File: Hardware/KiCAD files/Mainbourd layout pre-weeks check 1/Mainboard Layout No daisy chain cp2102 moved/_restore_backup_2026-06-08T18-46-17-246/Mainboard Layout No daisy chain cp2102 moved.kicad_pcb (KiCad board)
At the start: 2 copper layers, 207 x 174.8 mm, 107 parts, among them J1 JST_03, J11 Conn_01x04, J12 JST_06, J13 Conn_01x08, J14 Conn_01x08, J17 PINHD_1x8_Male, J18 PINHD_1x8_Male, J19 PINHD_1x8_Male, J2 Screw_Terminal_2_P5.00mm, J20 PINHD_1x8_Male, J22 PINHD_1x8_Male, J23 PINHD_1x8_Male, J24 PINHD_1x8_Male, J25 Conn_01x04, J26 Conn_01x04, J27 Conn_01x04, J28 PINHD_1x8_Male, J3 Screw_Terminal_2_P3.50mm, J30 USB-A1VSB6, J31 JST_03, J32 USB-A1VSB6, J34 JST_03, J35 JST_03, J36 JST_03, J37 JST_03, J38 JST_03, J4 JST_06, J5 Conn_01x04, J6 JST_06, J7 JST_06, J9 Conn_01x10, Q1 BS170, Q2 2DD1664, SW1 210-4MS, SW2 210-4MS, SW3 210-4MS, SW4 210-4MS, SW8 Push_Button, SW9 Push_Button, U1 CP2102-GM, U12 ESP32-S3-WROOM-1, U2 PCA9534PW_118, U4 PCA9534PW_118

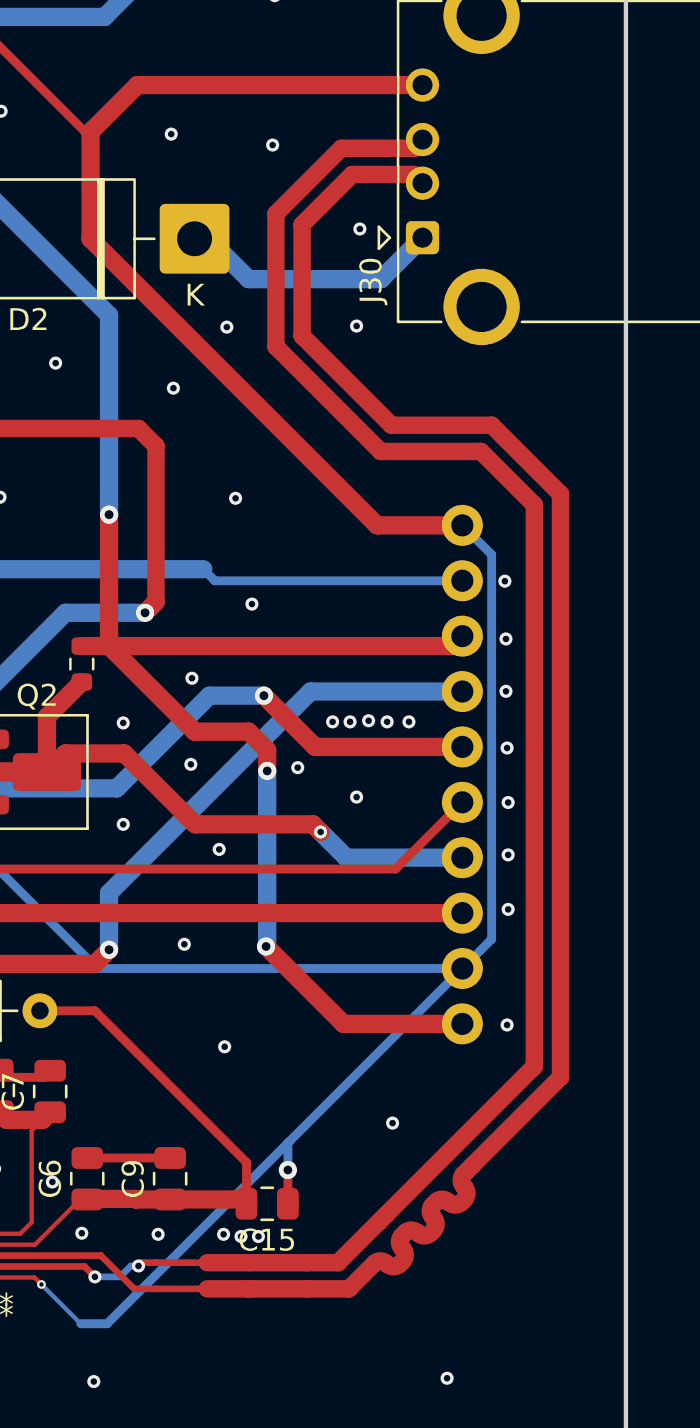
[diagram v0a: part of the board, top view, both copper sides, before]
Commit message: V2 mainboard
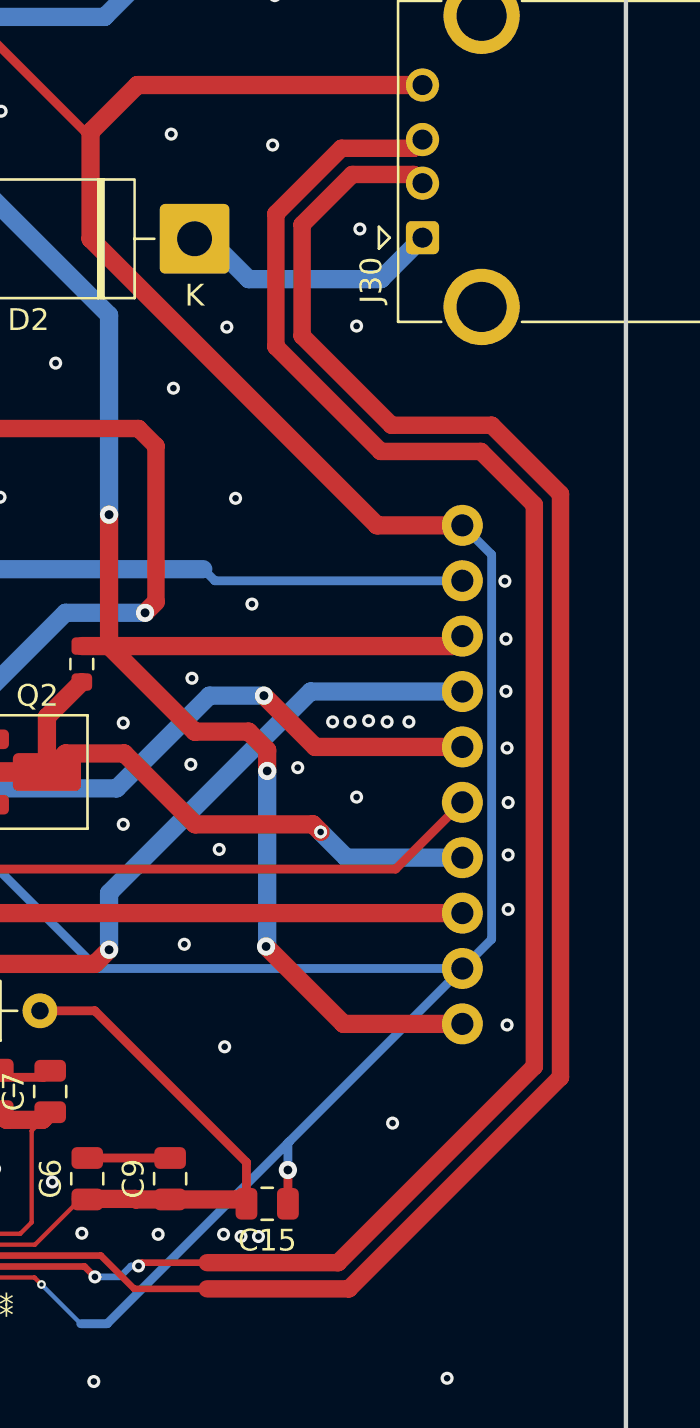
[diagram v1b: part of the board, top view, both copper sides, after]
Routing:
- net Prog_D-: track 87.3 -> 84.5 mm
